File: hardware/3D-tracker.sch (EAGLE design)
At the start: 24 parts, among them IC1 TS4231, IC2 NRF52840, IC3 MIC5233-3.3YS, Q1 DMP2035U

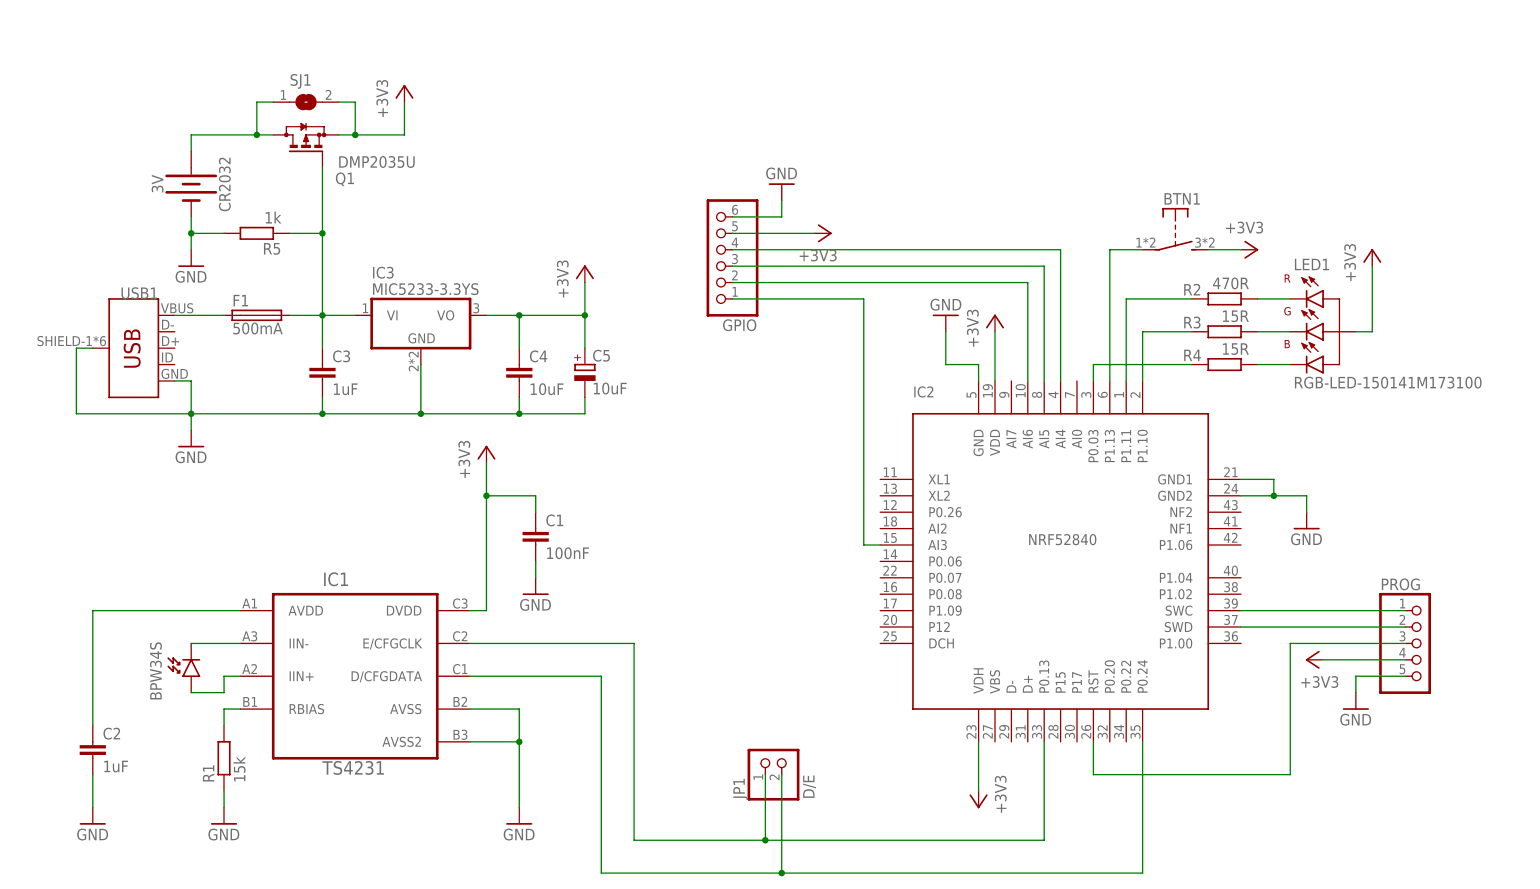
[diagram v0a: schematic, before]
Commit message: Update electrical scheme, add gerber file, add hw images
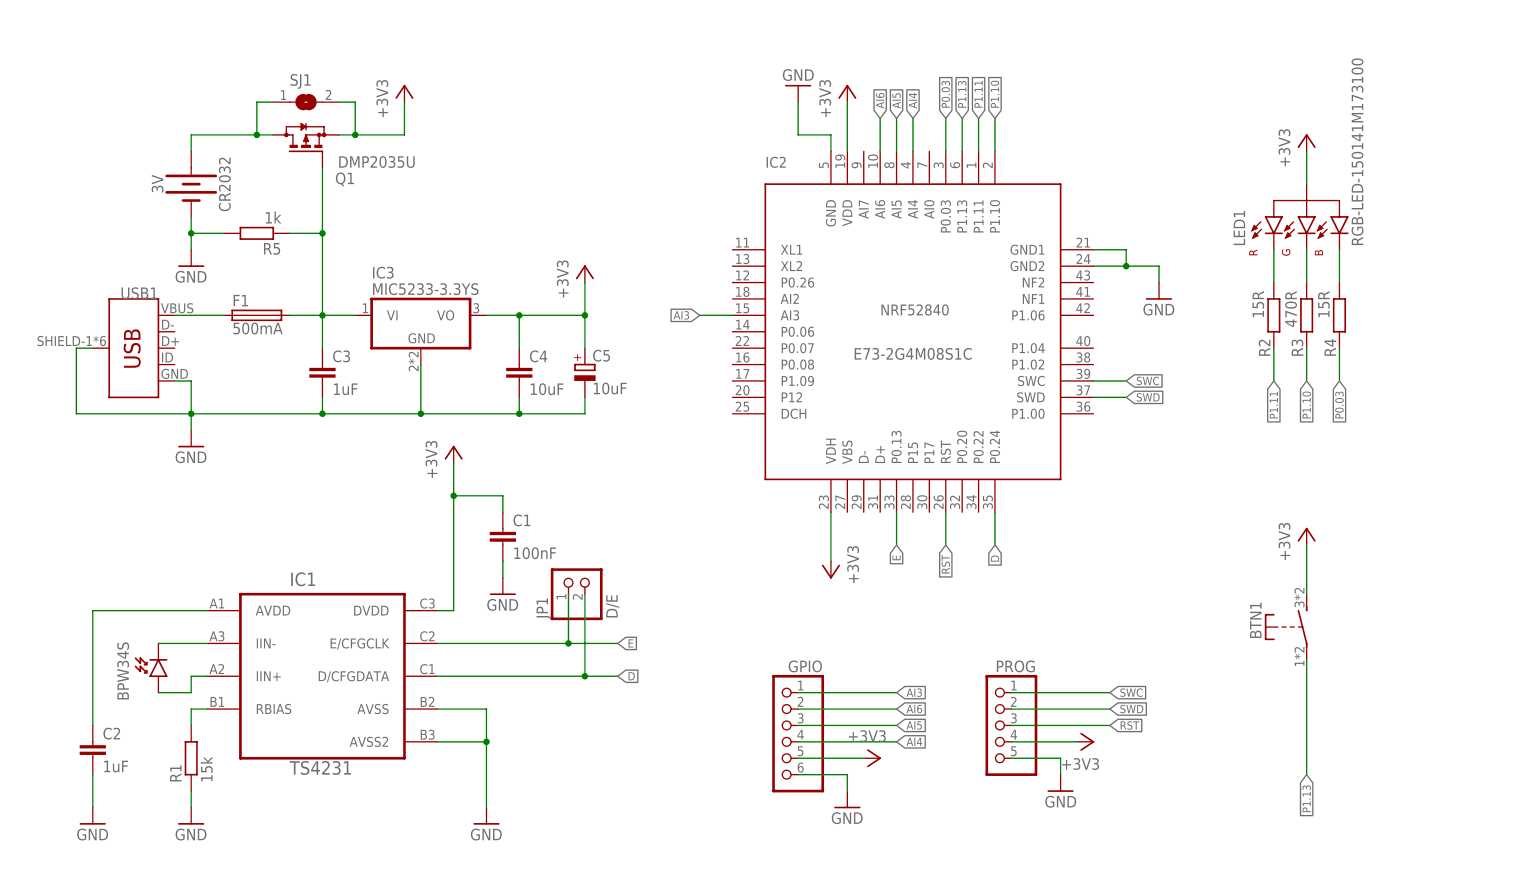
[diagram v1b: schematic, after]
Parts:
- R2: value 470R -> 15R
- R3: value 15R -> 470R
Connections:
- net N$14 renamed P1.13
- net N$2 renamed P1.11
- net N$4 renamed P1.10
- net N$5 renamed P0.03
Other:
- note added: "E73-2G4M08S1C"
- moved on the sheet: BPW34S, BTN1, C1, GPIO, IC1, IC2, JP1, LED1, PROG, R1, R2, R3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
